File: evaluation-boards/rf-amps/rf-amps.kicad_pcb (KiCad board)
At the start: 4 copper layers, 23 x 37 mm, 22 parts, among them J1 Conn_01x02, J2 Conn_01x02, J3 CONN_01X03, J4 CONN_COAXIAL, J5 CONN_COAXIAL, J6 CONN_COAXIAL, J7 CONN_COAXIAL, U1 BGB741L7ESD

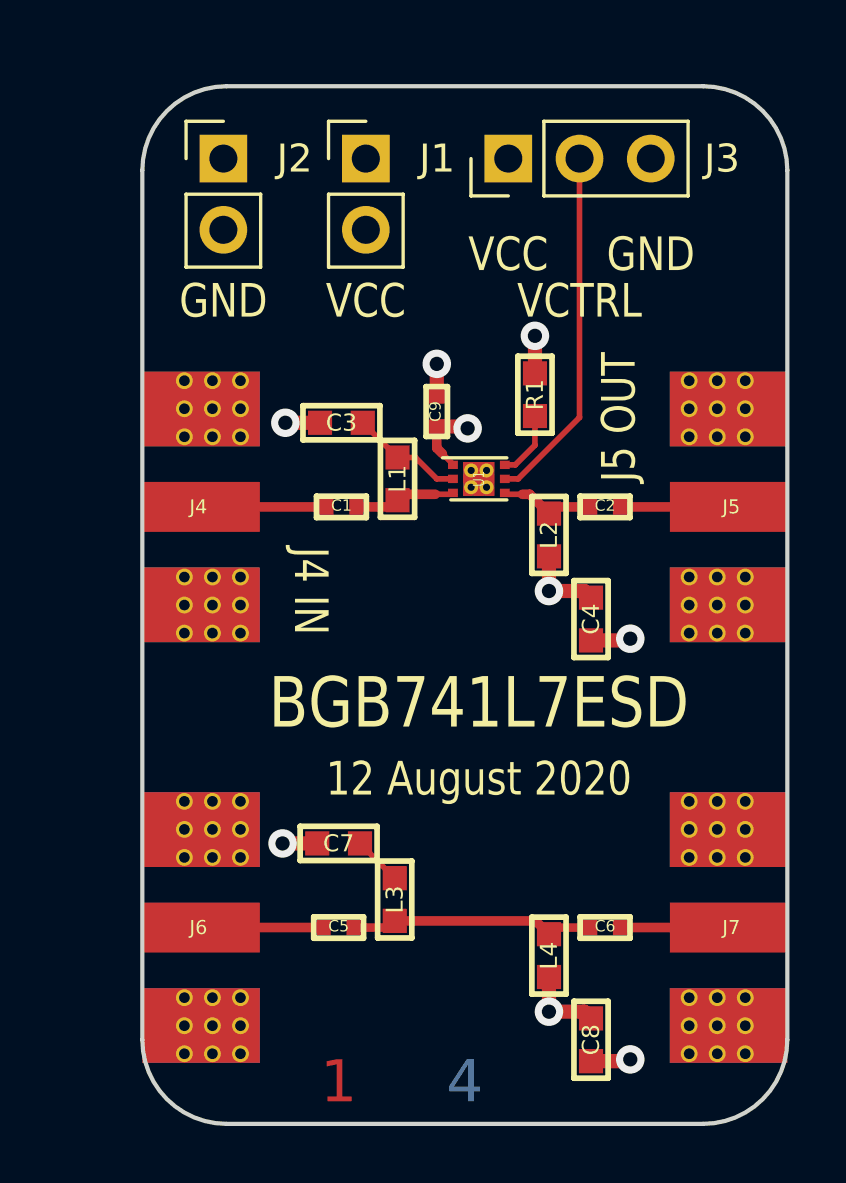
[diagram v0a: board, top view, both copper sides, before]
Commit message: Update rf-amps board
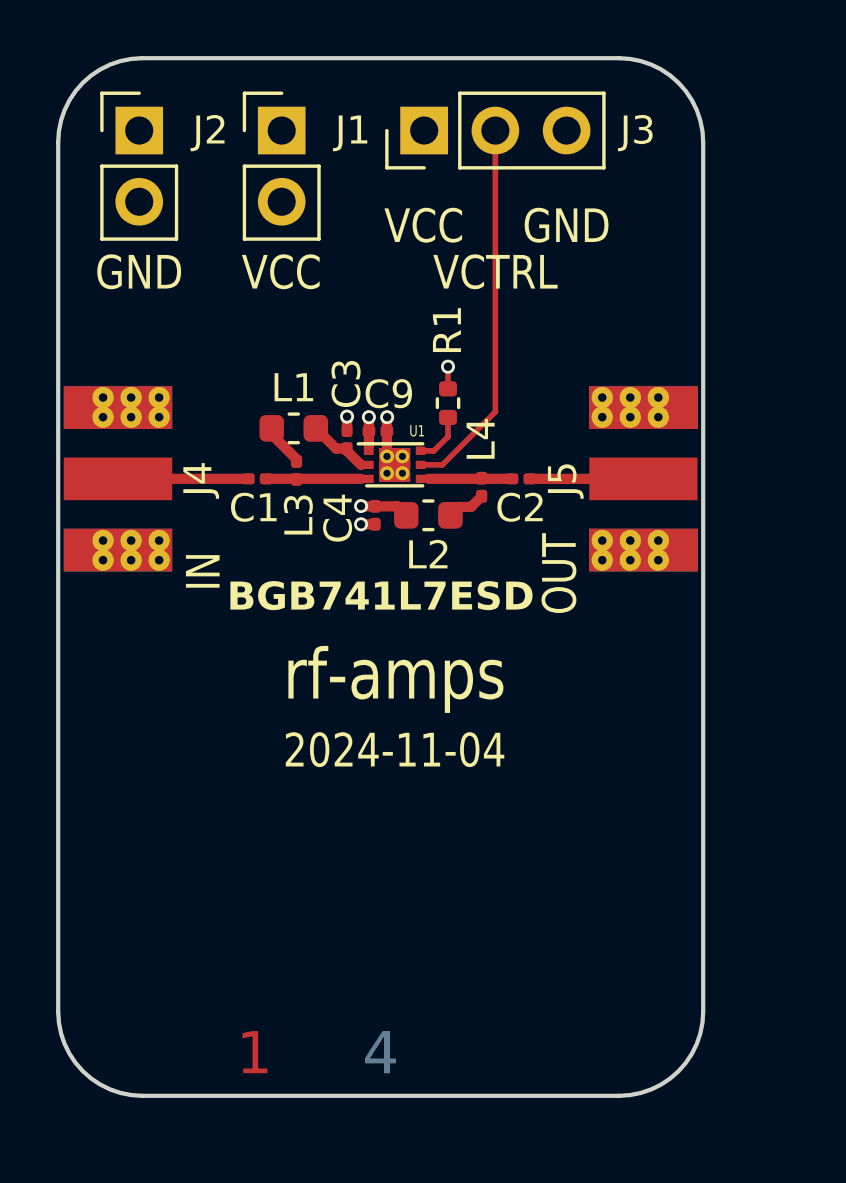
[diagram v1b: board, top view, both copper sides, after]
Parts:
- removed C5, C6: 100nF, gsg-modules:0402
- removed C7, C8: 1uF, gsg-modules:0603
- removed J6, J7: CONN_COAXIAL, gsg-modules:SMA-73251-2120
- C1, C2, C9: value 100nF -> 1uF; footprint gsg-modules:0402 -> Capacitor_SMD:C_0201_0603Metric
- C3, C4: footprint gsg-modules:0603 -> Capacitor_SMD:C_0201_0603Metric
- J4, J5: footprint gsg-modules:SMA-73251-2120 -> sma-variants:Linx_SMA_CONSMA003.062
- L1, L2: value 10uH -> 47uH; footprint gsg-modules:0603 -> Inductor_SMD:L_0603_1608Metric
- L3, L4: value 10uH -> 33nH; footprint gsg-modules:0603 -> Inductor_SMD:L_0201_0603Metric
- R1: footprint gsg-modules:0603 -> Resistor_SMD:R_0402_1005Metric
- moved L4 16.9 mm to (145.1, 80.3)
- moved L3 15.7 mm to (138.5, 79.7)
- moved C4 8.54 mm to (141.3, 81.3)
- moved L2 4.36 mm to (143.2, 81.3), turned to 180 degrees
- moved L1 4.11 mm to (138.4, 78.2), turned to 0 degrees
- moved C1 3.16 mm to (137.1, 80.0)
- moved C2 3.16 mm to (146.5, 80.0)
- moved J1 3.16 mm to (138.0, 67.6)
- moved J2 3.16 mm to (132.9, 67.6)
- moved J3 3.16 mm to (143.1, 67.6)
- moved J4 3.16 mm to (130.0, 80.0)
- moved J5 3.16 mm to (153.0, 80.0)
- moved R1 3.11 mm to (143.9, 77.3)
- moved U1 3.04 mm to (142.0, 79.5)
- moved C9 2.21 mm to (141.4, 78.3), turned to 180 degrees
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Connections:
- C1 pad 1: Net-(C1-Pad1) -> Net-(U1-RFIN)
- C2 pad 2: Net-(C2-Pad2) -> Net-(U1-RFOUT)
- L1 pad 1: Net-(C1-Pad1) -> Net-(L1-Pad1)
- L2 pad 1: Net-(C2-Pad2) -> Net-(L2-Pad1)
- L3 pad 1: Net-(C5-Pad1) -> Net-(U1-RFIN)
- L3 pad 2: Net-(C7-Pad2) -> Net-(L1-Pad1)
- L4 pad 1: Net-(C5-Pad1) -> Net-(U1-RFOUT)
- L4 pad 2: VCC -> Net-(L2-Pad1)
- U1 pad 3: Net-(C1-Pad1) -> Net-(U1-RFIN)
- U1 pad 4: Net-(C2-Pad2) -> Net-(U1-RFOUT)
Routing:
- net Net-(C5-Pad1): track 8.83 -> 0.00 mm
- net VCC: track 9.74 -> 3.57 mm, vias 4 -> 3
- net Net-(C5-Pad2): track 4.37 -> 0.00 mm
- net GND: track 6.49 -> 2.41 mm, vias 5 -> 3
- net Net-(C6-Pad1): track 3.87 -> 0.00 mm
- net Net-(C1-Pad1): track 3.70 -> 0.00 mm
- net Net-(C2-Pad2): track 3.50 -> 0.00 mm
- net Net-(U1-RFIN): track 0.00 -> 3.40 mm
- net Net-(U1-RFOUT): track 0.00 -> 3.00 mm
- net Net-(U1-BIAS): track 4.04 -> 2.21 mm
- net Net-(C7-Pad2): track 1.75 -> 0.00 mm
- net Net-(L1-Pad1): track 0.00 -> 1.55 mm
- net Net-(L2-Pad1): track 0.00 -> 1.39 mm
- net Net-(J3-Pin_2): track 12.8 -> 13.5 mm
- net Net-(U1-ADJ): track 2.40 -> 1.87 mm
- added copper zone on In1.Cu, net GND
- added copper zone on In2.Cu, net VCC
- removed copper zone on C2.Cu, net GND
- removed copper zone on C3.Cu, net VCC
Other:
- net class Default removed
- board text added: "2024-11-04"
- board text added: "IN"
- board text added: "OUT"
- board text added: "rf-amps"
- board text removed: "12 August 2020"
- board text removed: "J4 IN"
- board text removed: "J5 OUT"
